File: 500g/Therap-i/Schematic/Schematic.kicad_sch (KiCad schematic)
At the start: 13 parts, among them IC1 TC78H653FTG,EL, U1 Teensy4.1, U2 IFX27001TFV50, U3 IFX27001TFV50

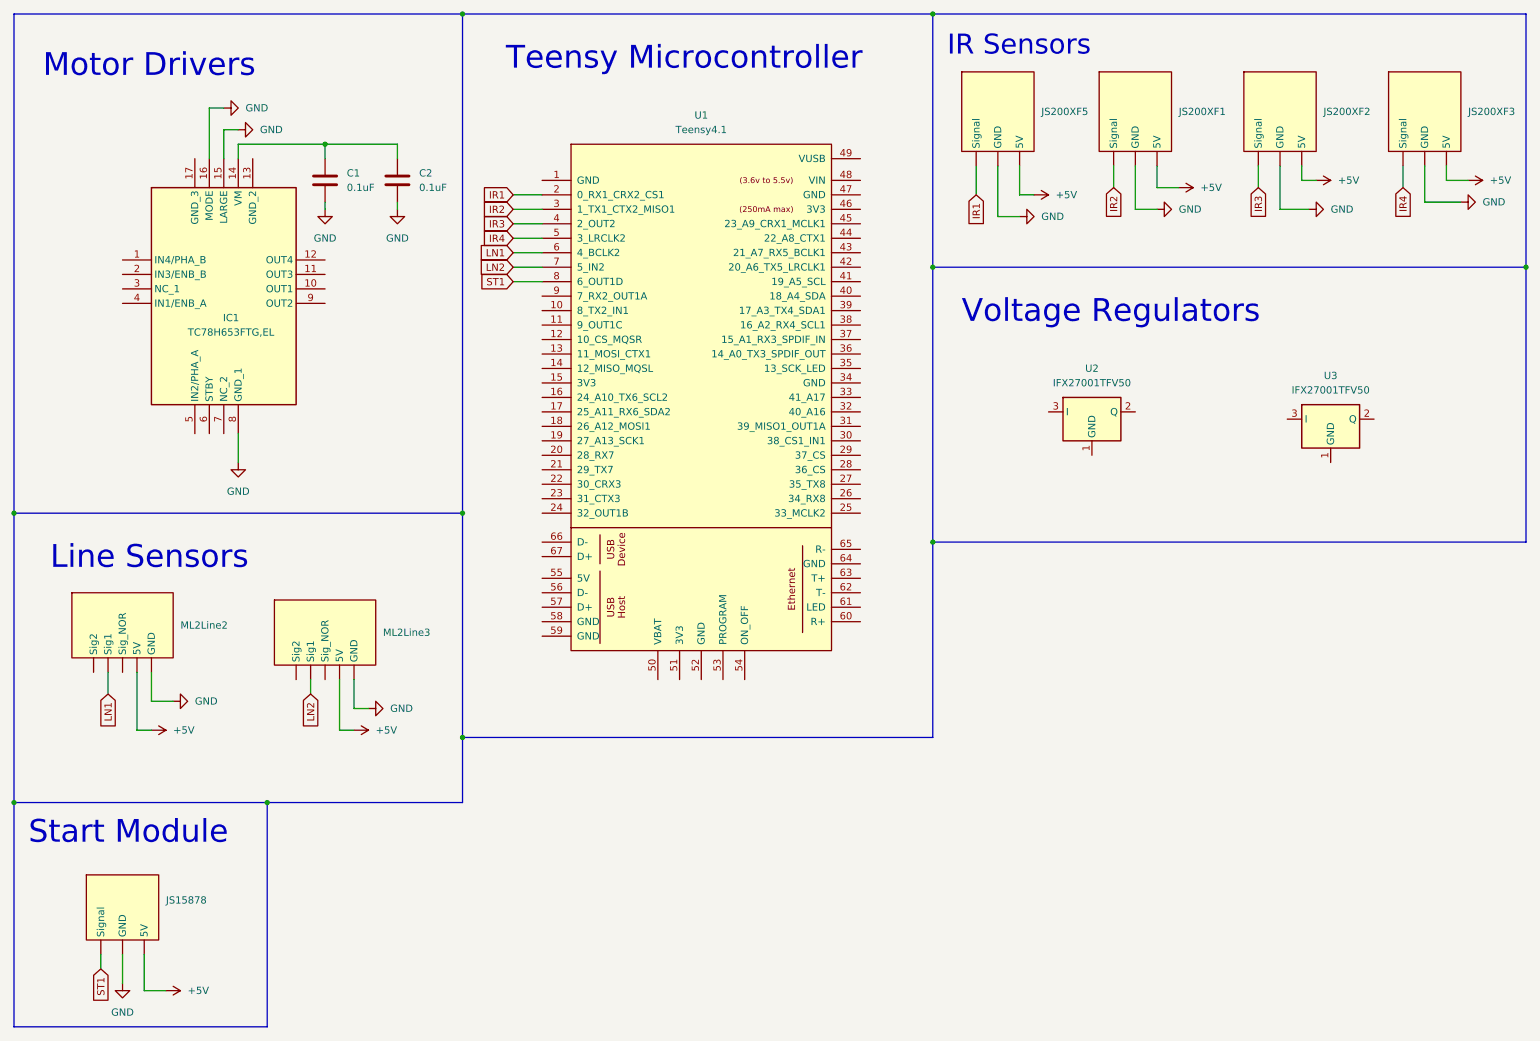
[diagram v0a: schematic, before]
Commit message: voltage regulator and battery
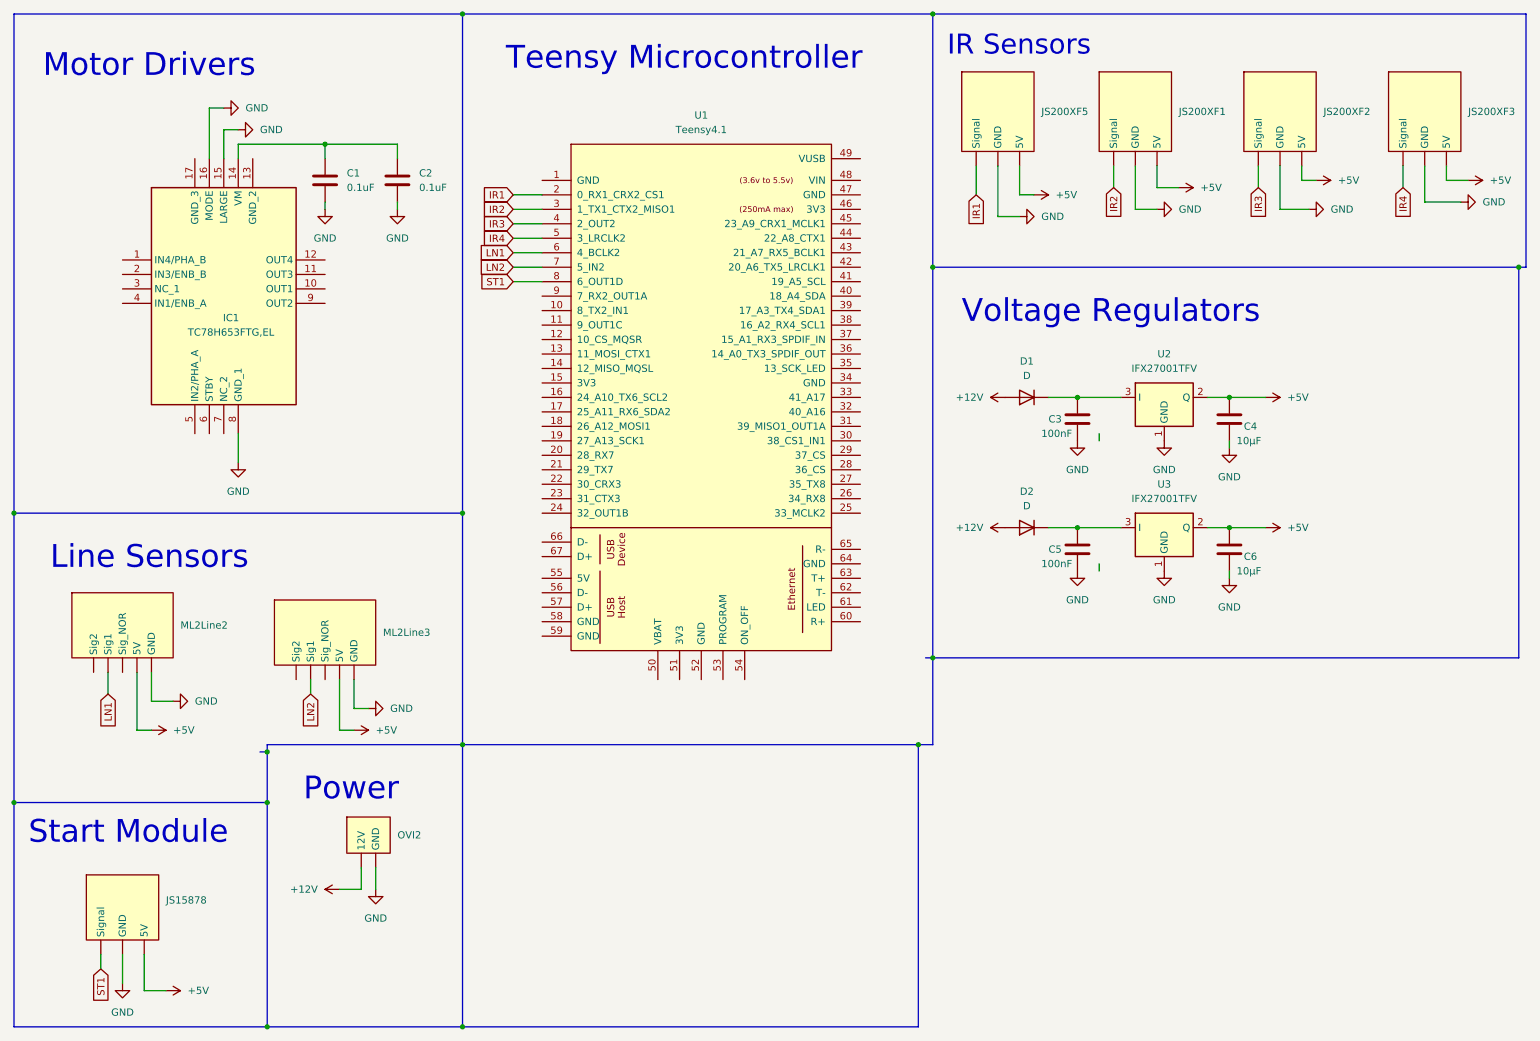
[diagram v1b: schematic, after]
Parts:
- added C3, C5: 100nF, symbol Device:C
- added C4, C6: 10µF, symbol Device:C
- added D1, D2: D, symbol Device:D
- added OVI2: ~, symbol power:OVI
- U2, U3: value IFX27001TFV50 -> IFX27001TFV
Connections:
- net +5V: now also U2.2 (Q), U3.2 (Q), C4.1, C6.1
- net GND: now also U2.1 (GND), U3.1 (GND), C3.2, C4.2, C5.2, C6.2, OVI2. (GND)
- net at U2.3 (I): now also C3.1, D1.1 (K)
- net at U3.3 (I): now also C5.1, D2.1 (K)
- new net +12V: D1.2 (A), D2.2 (A), OVI2. (GND)
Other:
- note added: "Power"
- moved on the sheet: U2
